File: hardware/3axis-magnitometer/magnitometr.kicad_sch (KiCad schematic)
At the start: 11 parts, among them U5 qmc5883l

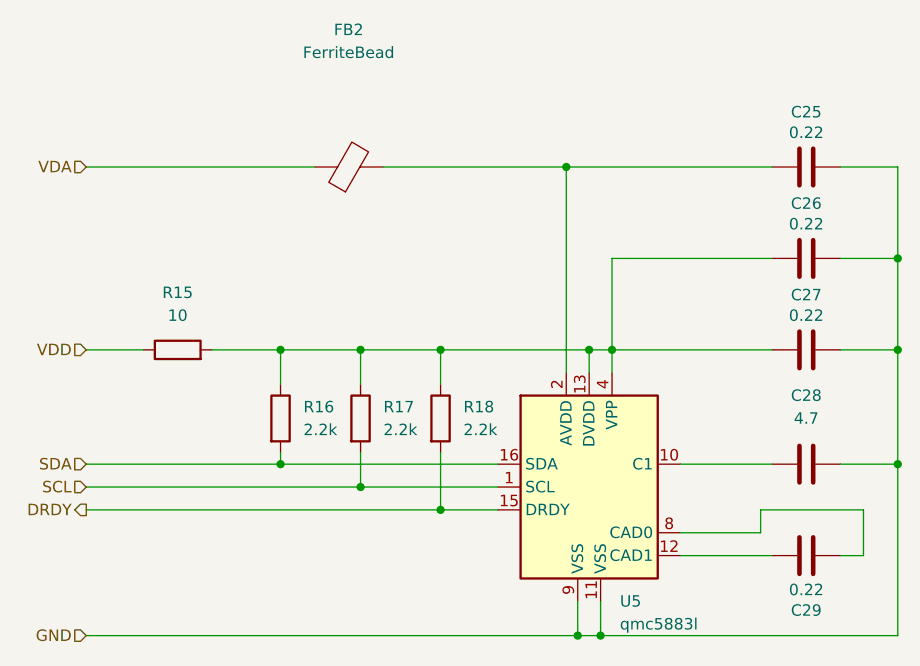
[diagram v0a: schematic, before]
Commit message: Add files via upload
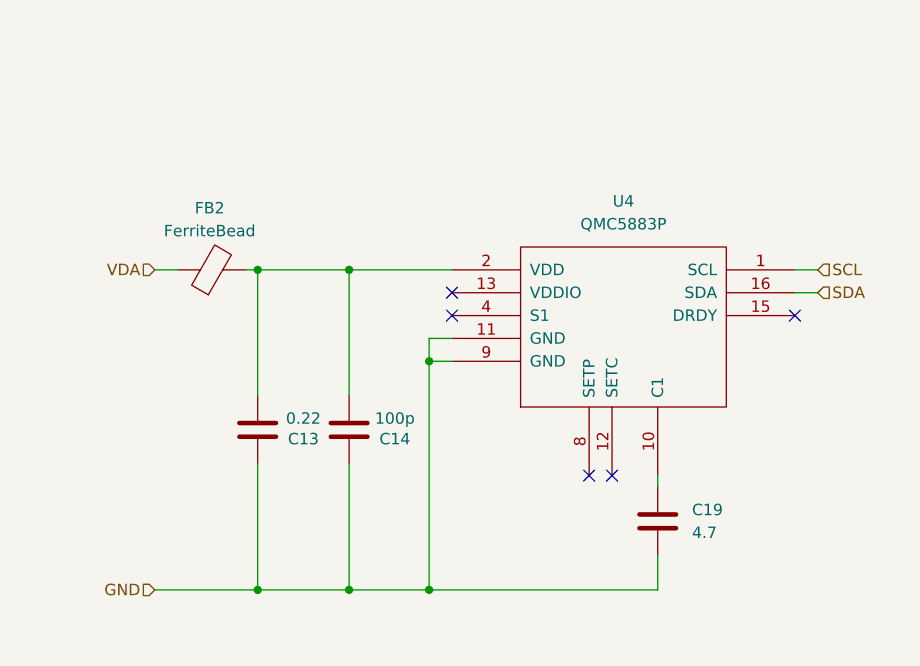
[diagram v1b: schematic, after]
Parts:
- removed C25, C26, C27, C29: 0.22, Capacitor_SMD:C_0805_2012Metric, symbol Device:C
- removed C28: 4.7, Capacitor_SMD:C_0805_2012Metric, symbol Device:C
- removed R15: 10, Resistor_SMD:R_0805_2012Metric, symbol Device:R
- removed R16, R17, R18: 2.2k, Resistor_SMD:R_0805_2012Metric, symbol Device:R
- removed U5: qmc5883l, Package_LGA:LGA-16_3x3mm_P0.5mm, symbol Sensor_Magnetic:qmc5883l
- added C13: 0.22, Capacitor_SMD:C_0805_2012Metric, symbol Device:C
- added C14: 100p, Capacitor_SMD:C_0805_2012Metric, symbol Device:C
- added C19: 4.7, Capacitor_SMD:C_0805_2012Metric, symbol Device:C
- added U4: QMC5883P, MODULE, symbol common:QMC5883P
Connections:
- net GND: now also C13.2, C14.2, C19.2, U4.11 (GND), U4.9 (GND)
- net SCL: now also U4.1 (SCL)
- net SDA: now also U4.16 (SDA)
- net at FB2.2: now also C13.1, C14.1, U4.2 (VDD)
- new net: C19.1, U4.10 (C1)
- no-connect marks 0 -> 5
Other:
- moved on the sheet: FB2
